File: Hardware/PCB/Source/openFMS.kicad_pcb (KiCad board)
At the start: 2 copper layers, 30 x 70 mm, 44 parts, among them U1 STM32F030F4Px, X1 8 MHz

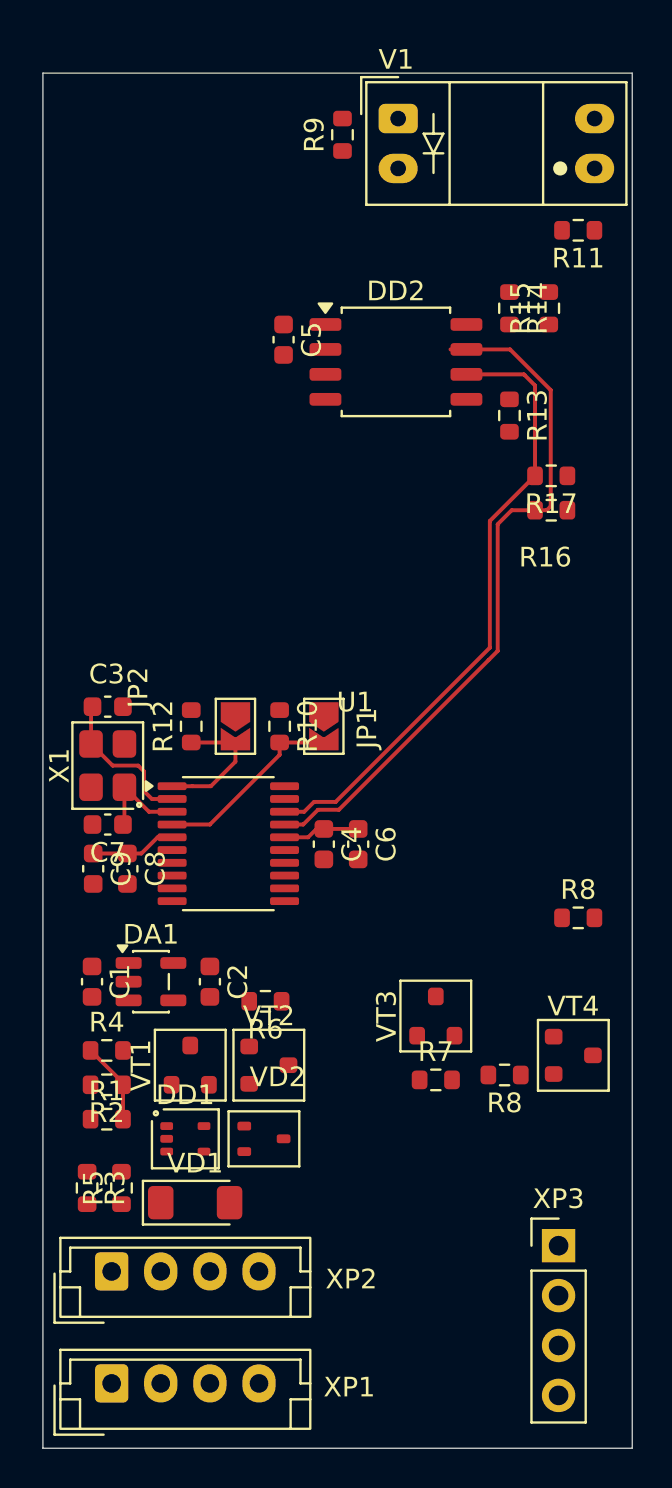
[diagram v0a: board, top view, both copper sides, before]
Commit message: WIP: routing
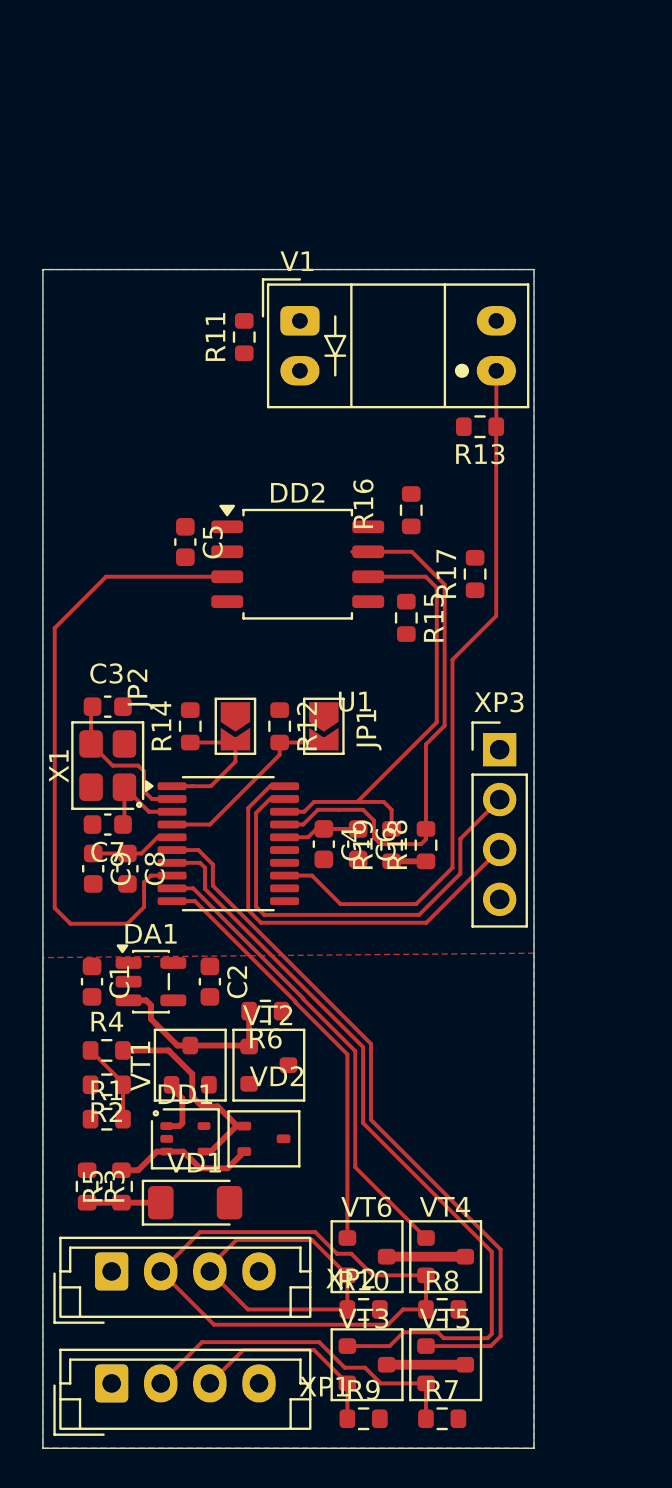
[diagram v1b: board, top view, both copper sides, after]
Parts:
- removed the R8 at (140.0, 98.0)
- added R18: 2k, Resistor_SMD:R_0603_1608Metric, F.Cu at (136.0, 86.3)
- added R19: 2k, Resistor_SMD:R_0603_1608Metric, F.Cu at (134.2, 86.3)
- added VT5: BSS138L, Package_TO_SOT_SMD_AKL:SOT-23, F.Cu at (133.0, 112.8)
- added VT6: BSS138L, Package_TO_SOT_SMD_AKL:SOT-23, F.Cu at (133.0, 107.2)
- R11: value 10k -> 110
- R16, R17: value 2k -> 10k
- R9: value 110 -> 10k
- moved R9 65.4 mm to (132.8, 115.5), turned to 0 degrees
- moved R10 30.0 mm to (132.8, 109.9), turned to 0 degrees
- moved R14 26.8 mm to (124.0, 80.2), turned to 90 degrees
- moved XP3 25.4 mm to (139.8, 81.4)
- moved R8 21.1 mm to (136.8, 109.9)
- moved R11 17.8 mm to (126.8, 60.4), turned to 90 degrees
- moved VT3 17.8 mm to (137.0, 112.8), turned to 0 degrees
- moved R15 17.3 mm to (135.0, 74.7), turned to -90 degrees
- moved R7 17.3 mm to (136.8, 115.5)
- moved VT4 12.1 mm to (137.0, 107.2)
- moved C5 11.4 mm to (123.8, 70.9)
- moved DD2 11.4 mm to (129.5, 72.0)
- moved V1 11.4 mm to (129.6, 59.6)
- moved R16 7.12 mm to (135.2, 69.2), turned to 90 degrees
- moved R17 6.33 mm to (138.5, 72.5), turned to 90 degrees
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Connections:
- R10 pad 1: +3V3 -> /PA4_SIG
- R10 pad 2: /NRST -> GND
- R11 pad 1: /PHOTO_OUT -> +3V3
- R11 pad 2: +3V3 -> Net-(R11-Pad2)
- R12 pad 1: /BOOT -> +3V3
- R12 pad 2: GND -> /NRST
- R13 pad 1: Net-(DD2-PGO) -> /PHOTO_OUT
- R13 pad 2: GND -> +3V3
- R14 pad 1: +3V3 -> /BOOT
- R14 pad 2: Net-(DD2-DIR) -> GND
- R15 pad 1: Net-(DD2-DIR) -> Net-(DD2-PGO)
- R16 pad 2: /I2C_SCL -> Net-(DD2-DIR)
- R17 pad 1: +3V3 -> Net-(DD2-DIR)
- R17 pad 2: /I2C_SDA -> GND
- R8 pad 1: /FILAMENT_SENS -> /PA3_SIG
- R9 pad 1: +3V3 -> /FILAMENT_SENS
- R9 pad 2: Net-(R9-Pad2) -> GND
- U1 pad 11: /PA5 -> unconnected-(U1-PA5-Pad11)
- U1 pad 14: /HALL_OUT -> unconnected-(U1-PB1-Pad14)
- U1 pad 8: unconnected-(U1-PA2-Pad8) -> /HALL_OUT
- U1 pad 9: unconnected-(U1-PA3-Pad9) -> /PA3
- V1 pad 1: Net-(R9-Pad2) -> Net-(R11-Pad2)
- VT4 pad 1: /FILAMENT_SIG -> /PA3
- VT4 pad 2: /FILAMENT_SENS -> /PA3_SIG
- XP2 pad 2: /PA4 -> /PA3_SIG
- XP2 pad 3: /PA5 -> /PA4_SIG
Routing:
- net /FILAMENT_SIG: track 0.00 -> 39.4 mm
- net /MOTION_SIG: track 0.00 -> 36.5 mm
- net /PHOTO_OUT: track 0.00 -> 36.1 mm
- net /HALL_OUT: track 0.00 -> 32.2 mm
- net /PA3_SIG: track 0.00 -> 31.9 mm
- net /PA3: track 0.00 -> 23.8 mm
- net /SWDIO: track 0.00 -> 22.6 mm
- net /SWCLK: track 0.00 -> 22.1 mm
- net /PA4: track 0.00 -> 21.5 mm
- net /PA4_SIG: track 0.00 -> 18.1 mm
- net /MOTION_SENS: track 0.00 -> 17.0 mm
- net Net-(DD1--): track 0.00 -> 11.0 mm
- net /FILAMENT_SENS: track 0.00 -> 10.2 mm
- net Net-(DA1-EN): track 0.00 -> 9.32 mm
- net /I2C_SDA: track 31.9 -> 23.1 mm
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- added copper zone on B.Cu, net GND
- added copper zone on F.Cu, net VCC
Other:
- board size 30 x 70 mm -> 25 x 60 mm
